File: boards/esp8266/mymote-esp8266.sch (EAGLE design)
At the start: 36 parts, among them IC1 ESP-12-SMD, IC31 MCP73831/OT, IC32 MCP1703CB

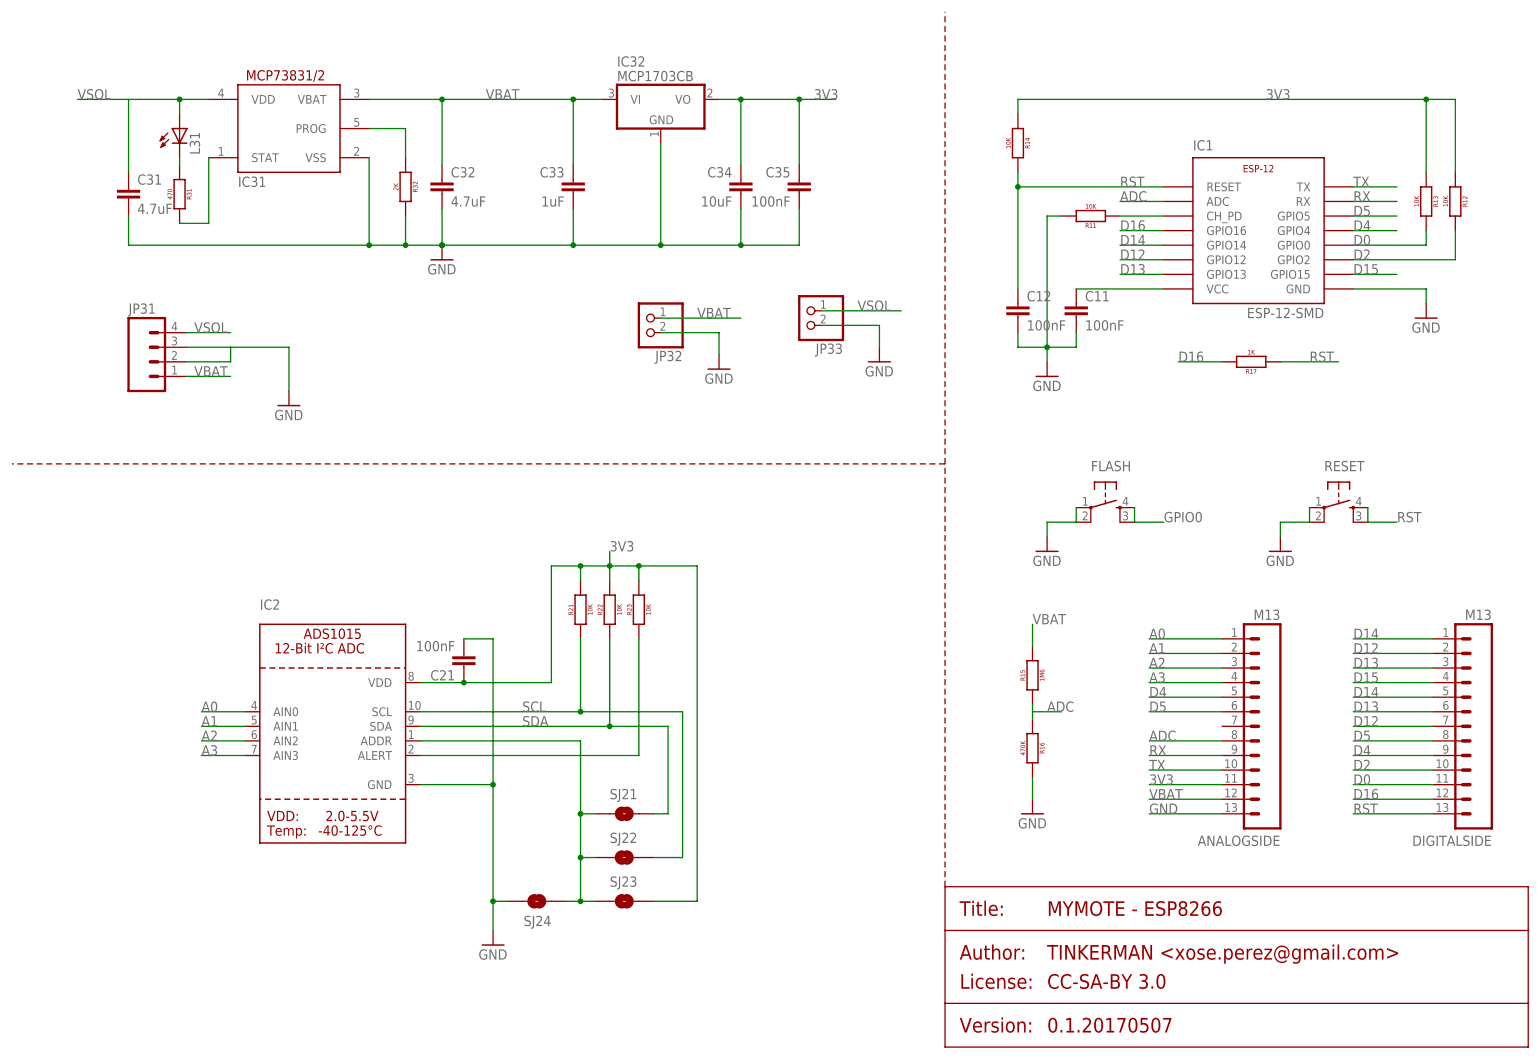
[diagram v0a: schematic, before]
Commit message: Relay board and oter small changes
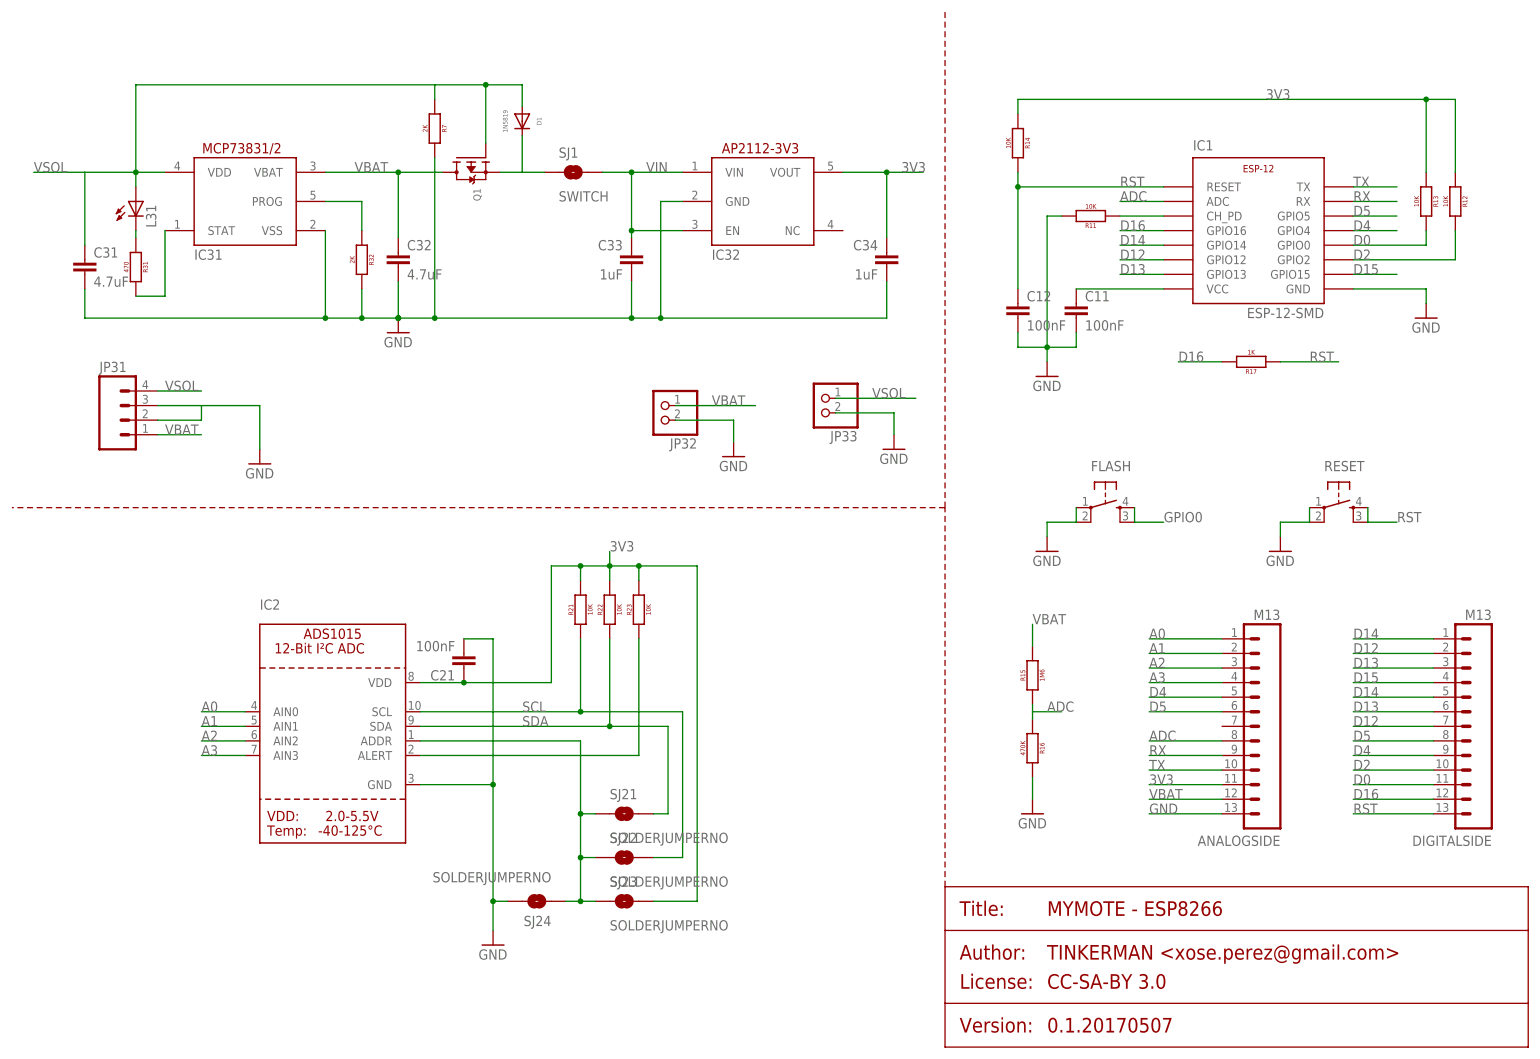
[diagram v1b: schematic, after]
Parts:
- removed C35: 100nF, xose:C-EU0805
- added D1: 1N5819, xose:DIODE-SMD
- added Q1: (no value), xose:MOSFET-PWIDE
- added R7: 2K, xose:RESISTOR0805
- added SJ1: SWITCH, xose:SOLDERJUMPERTRACE-PTH
- C34: value 10uF -> 1uF
- IC32: value MCP1703CB -> AP2112-3V3; device xose:MCP1703CB -> xose:AP2112-3V3
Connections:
- new net N$9: D1.C, Q1.S, SJ1.1
- new net VIN: C33.1, IC32.EN, IC32.VIN, SJ1.2
- net 3V3: now also IC32.VOUT; no longer C35.1, IC32.VO
- net GND: now also R7.2; no longer C35.2
- net VBAT: now also Q1.D; no longer C33.1, IC32.VI
- net VSOL: now also D1.A, Q1.G, R7.1
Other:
- moved on the sheet: C31, C32, C33, C34, IC31, JP31, JP32, JP33, L31, R31, R32
